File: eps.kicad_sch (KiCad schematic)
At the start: 15 parts, among them J2 Conn_01x02_Pin, J3 Conn_01x02_Pin, J4 Conn_01x02_Pin

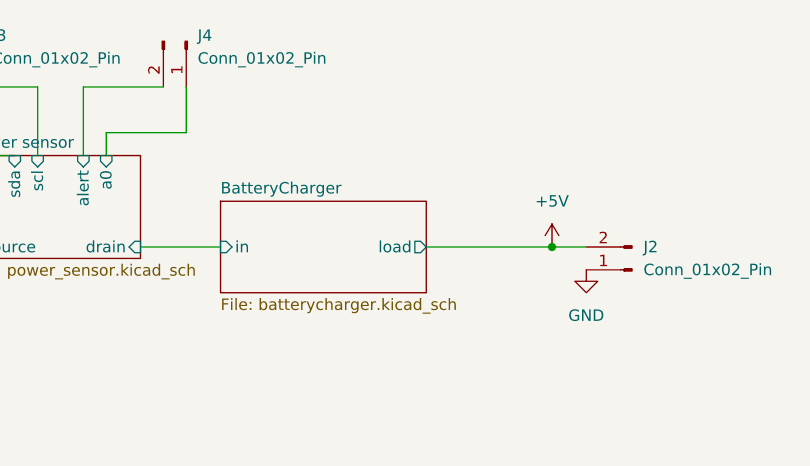
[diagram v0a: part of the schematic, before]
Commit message: Added
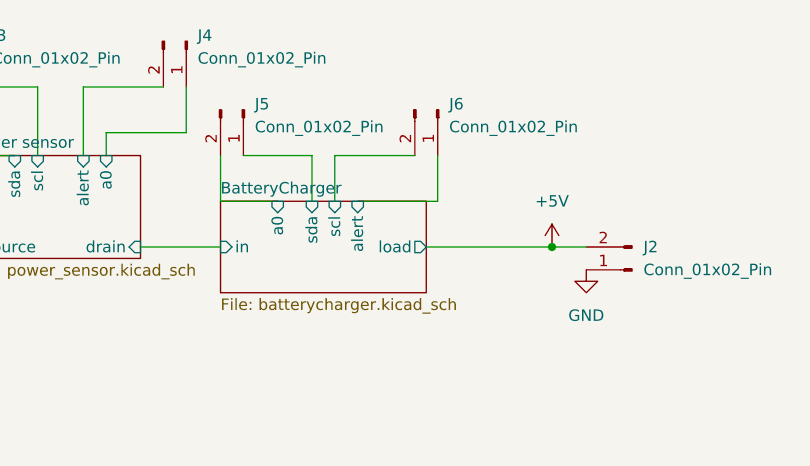
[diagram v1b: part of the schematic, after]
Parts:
- added J5, J6: Conn_01x02_Pin, Connector_PinHeader_2.00mm:PinHeader_1x02_P2.00mm_Vertical, symbol Connector:Conn_01x02_Pin
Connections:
- new net BatteryCharger/a0: J5.2 (Pin_2)
- new net BatteryCharger/alert: J6.1 (Pin_1)
- new net BatteryCharger/scl: J6.2 (Pin_2)
- new net BatteryCharger/sda: J5.1 (Pin_1)
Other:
- sheet BatteryCharger ports: added a0, alert, scl, sda; removed none

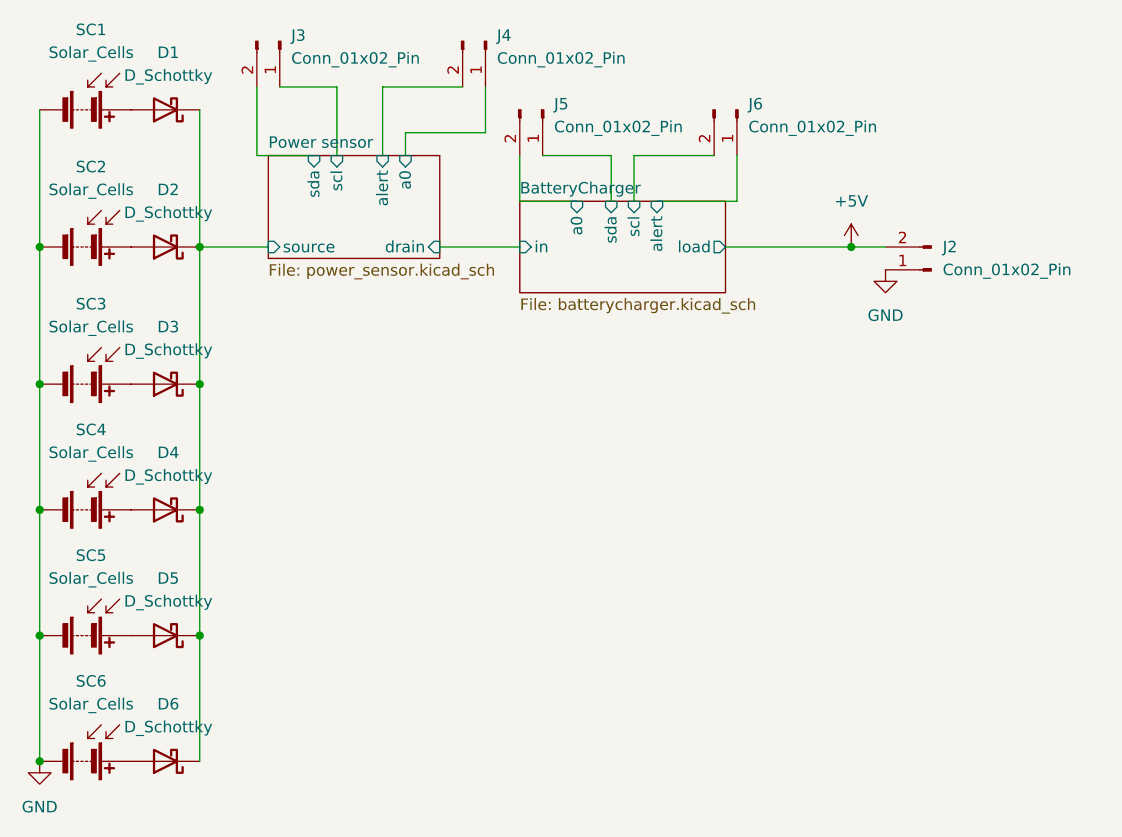
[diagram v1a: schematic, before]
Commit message: new design
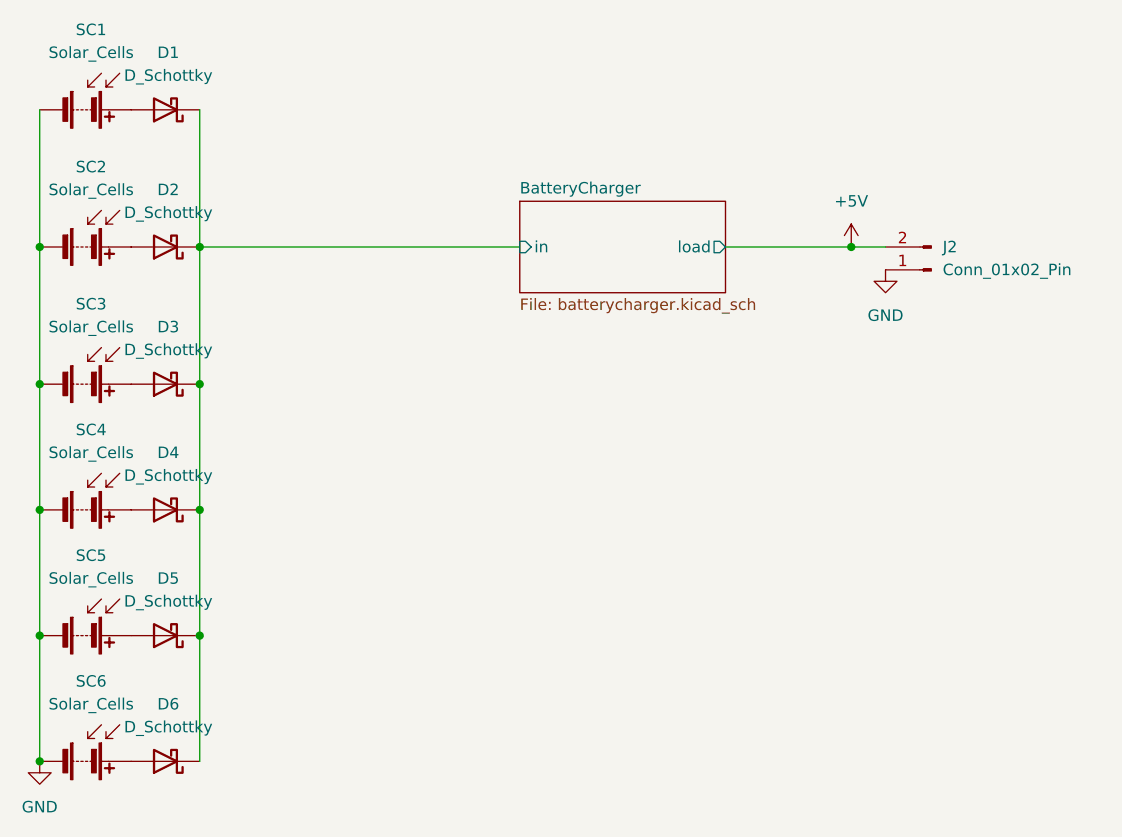
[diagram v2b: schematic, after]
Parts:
- removed J3, J4, J5, J6: Conn_01x02_Pin, Connector_PinHeader_2.00mm:PinHeader_1x02_P2.00mm_Vertical, symbol Connector:Conn_01x02_Pin
- J2, SC1, SC2, SC3, SC4, SC5, SC6: footprint Connector_PinHeader_2.00mm:PinHeader_1x02_P2.00mm_Vertical -> Connector_PinHeader_2.54mm:PinHeader_1x02_P2.54mm_Vertical
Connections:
- net Power sensor/source is gone; now on net BatteryCharger/in: D1.1 (K), D2.1 (K), D3.1 (K), D4.1 (K), D5.1 (K), D6.1 (K)
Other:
- removed sheet Power sensor
- sheet BatteryCharger ports: added none; removed a0, alert, scl, sda
